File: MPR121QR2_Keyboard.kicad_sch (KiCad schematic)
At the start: 71 parts, among them J1 USB_C_Receptacle_USB2.0_16P, SW1 SW_Push, SW2 SW_Push, U1 AP1117-33, U2 W25Q128JVS, U3 LM358D, U4 RP2040, U5 MPR121QR2, Y1 Crystal_GND24

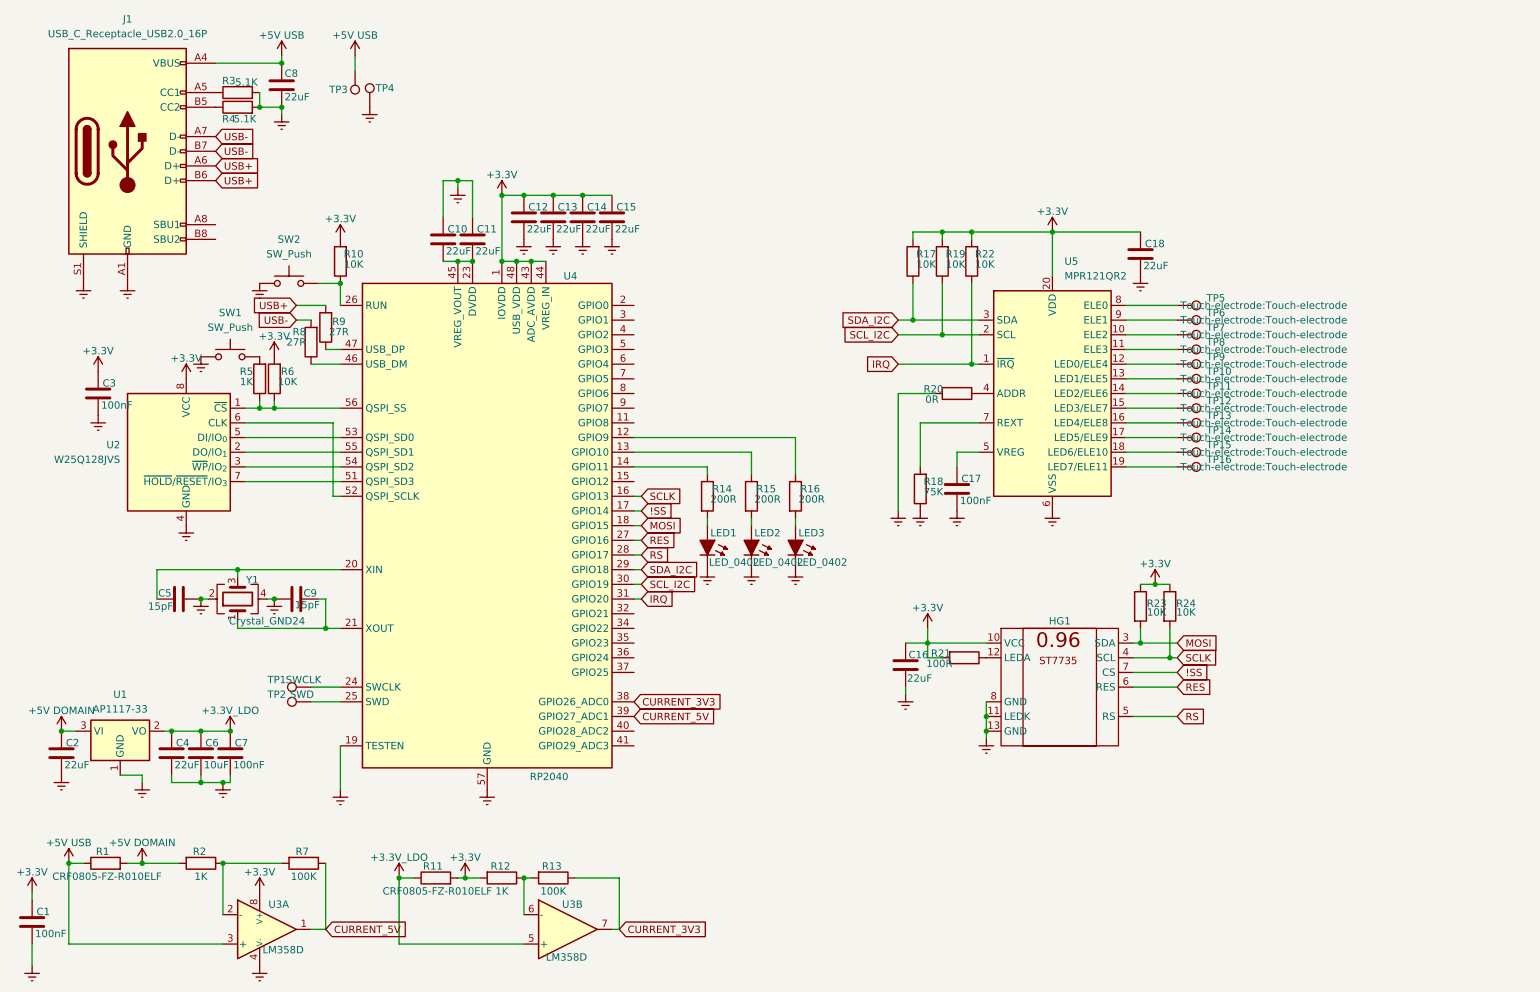
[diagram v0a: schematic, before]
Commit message: rev0
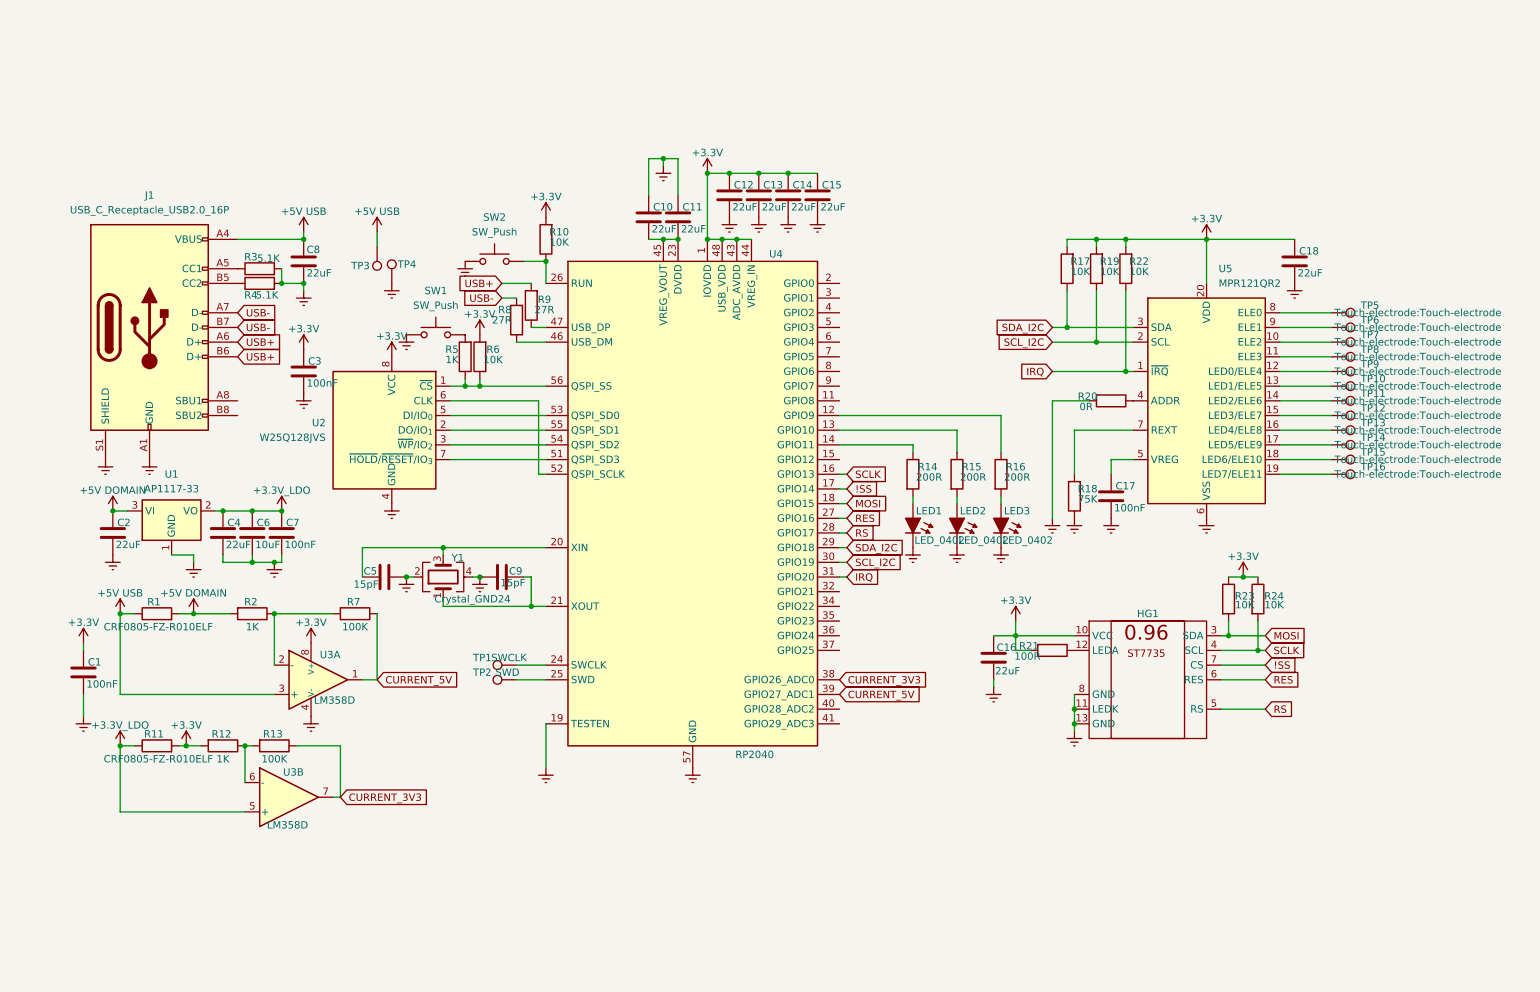
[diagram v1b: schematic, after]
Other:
- moved on the sheet: C1, C10, C11, C12, C13, C14, C15, C16, C17, C18, C2, C3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
